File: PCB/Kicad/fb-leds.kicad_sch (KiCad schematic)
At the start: 52 parts, among them Q1 MMBTA05L, Q2 MMBTA05L, Q3 MMBTA05L, Q4 MMBTA05L

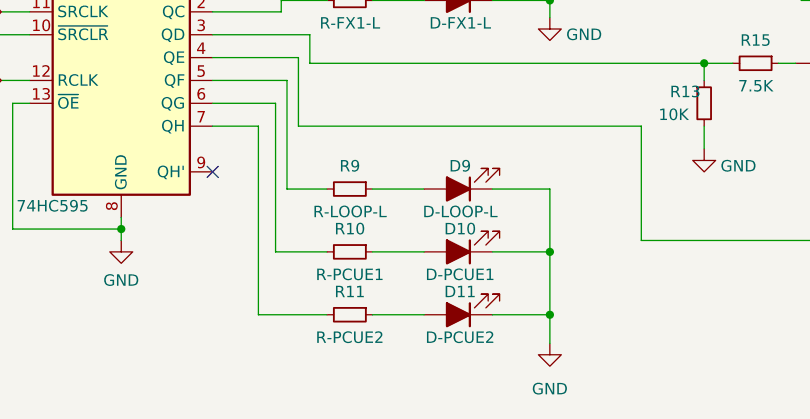
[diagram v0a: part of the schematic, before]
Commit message: routing WIP
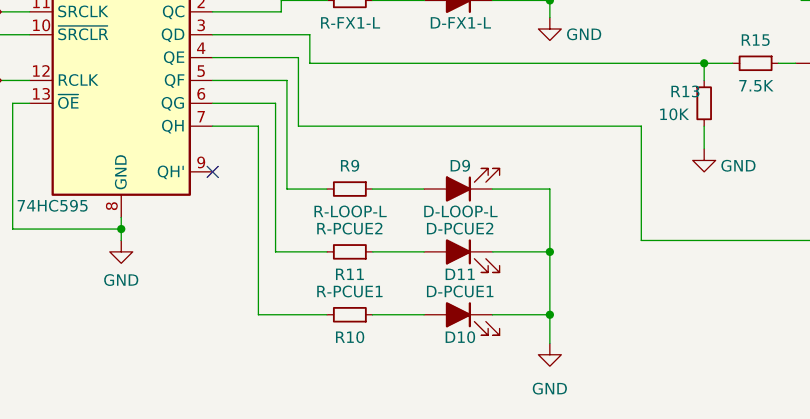
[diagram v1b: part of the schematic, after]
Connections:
- net at SR-FB-LEFT1.6 (QG): now also R11.2; no longer R10.2
- net at SR-FB-LEFT1.7 (QH): now also R10.2; no longer R11.2
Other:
- moved on the sheet: D10, D11, R10, R11
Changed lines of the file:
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@@
     (pin "2")
   )
-  (symbol (lib_id "Device:R_Small") (at 124.46 161.925 270) (unit 1)
-    (in_bom yes) (on_board yes)
-    (property "Reference" "R10" (id 0) (at 124.46 159.385 90))
-    (property "Value" "R-PCUE1" (id 1) (at 124.46 164.465 90))
+  (symbol (lib_id "Device:R_Small") (at 124.46 161.925 270) (mirror x) (unit 1)
+    (in_bom yes) (on_board yes)
+    (property "Reference" "R11" (id 0) (at 124.46 164.465 90))
+    (property "Value" "R-PCUE2" (id 1) (at 124.46 159.385 90))
     (property "Footprint" "Library:R_1206_3216Metric_Pad1.30x1.75mm_HandSolder" (id 2) (at 124.46 161.925 0)
       (effects (font (size 1.27 1.27)) hide)
@@
     (pin "2")
   )
-  (symbol (lib_id "Device:R_Small") (at 124.46 168.91 270) (unit 1)
-    (in_bom yes) (on_board yes)
-    (property "Reference" "R11" (id 0) (at 124.46 166.37 90))
-    (property "Value" "R-PCUE2" (id 1) (at 124.46 171.45 90))
+  (symbol (lib_id "Device:R_Small") (at 124.46 168.91 270) (mirror x) (unit 1)
+    (in_bom yes) (on_board yes)
+    (property "Reference" "R10" (id 0) (at 124.46 171.45 90))
+    (property "Value" "R-PCUE1" (id 1) (at 124.46 166.37 90))
     (property "Footprint" "Library:R_1206_3216Metric_Pad1.30x1.75mm_HandSolder" (id 2) (at 124.46 168.91 0)
       (effects (font (size 1.27 1.27)) hide)
@@
     (pin "2")
   )
-  (symbol (lib_id "Device:LED_Filled") (at 136.525 161.925 180) (unit 1)
-    (in_bom yes) (on_board yes)
-    (property "Reference" "D10" (id 0) (at 136.7155 159.385 0))
-    (property "Value" "D-PCUE1" (id 1) (at 136.7155 164.465 0))
+  (symbol (lib_id "Device:LED_Filled") (at 136.525 161.925 0) (mirror y) (unit 1)
+    (in_bom yes) (on_board yes)
+    (property "Reference" "D11" (id 0) (at 136.7155 164.465 0))
+    (property "Value" "D-PCUE2" (id 1) (at 136.7155 159.385 0))
     (property "Footprint" "Library:LED_1206_3216Metric_Pad1.42x1.75mm_HandSolder" (id 2) (at 136.525 161.925 0)
       (effects (font (size 1.27 1.27)) hide)
@@
     (pin "2")
   )
-  (symbol (lib_id "Device:LED_Filled") (at 136.525 168.91 180) (unit 1)
-    (in_bom yes) (on_board yes)
-    (property "Reference" "D11" (id 0) (at 136.7155 166.37 0))
-    (property "Value" "D-PCUE2" (id 1) (at 136.7155 171.45 0))
+  (symbol (lib_id "Device:LED_Filled") (at 136.525 168.91 0) (mirror y) (unit 1)
+    (in_bom yes) (on_board yes)
+    (property "Reference" "D10" (id 0) (at 136.7155 171.45 0))
+    (property "Value" "D-PCUE1" (id 1) (at 136.7155 166.37 0))
     (property "Footprint" "Library:LED_1206_3216Metric_Pad1.42x1.75mm_HandSolder" (id 2) (at 136.525 168.91 0)
       (effects (font (size 1.27 1.27)) hide)

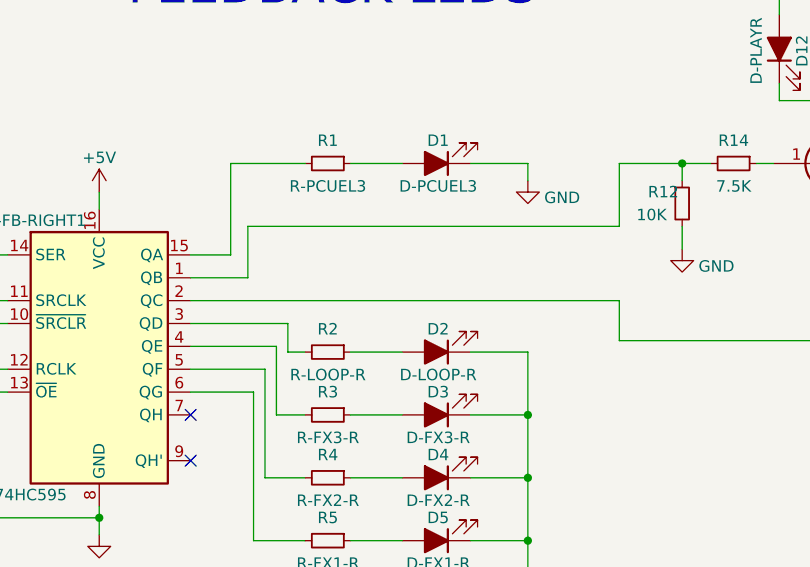
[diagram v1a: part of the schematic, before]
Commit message: routing WIP
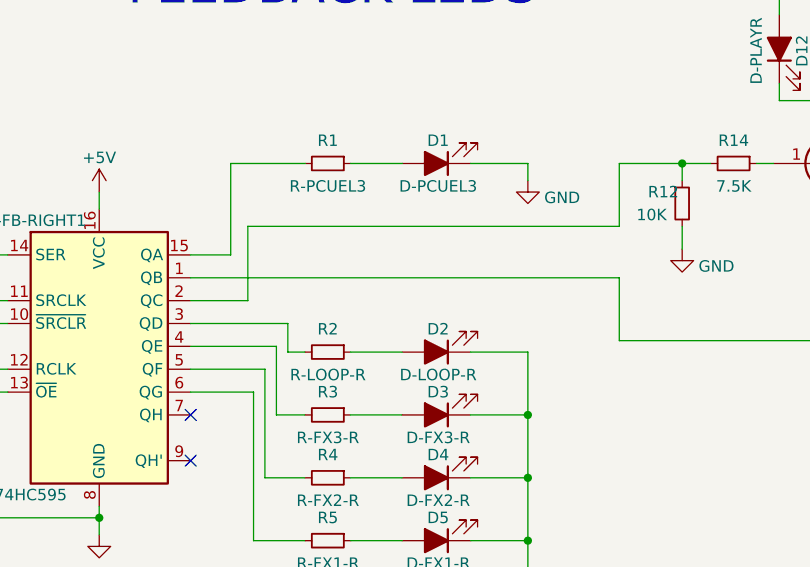
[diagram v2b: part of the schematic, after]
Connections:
- net at R12.1, R14.2: now also SR-FB-RIGHT1.2 (QC); no longer SR-FB-RIGHT1.1 (QB)
- net at R18.1, R20.2: now also SR-FB-RIGHT1.1 (QB); no longer SR-FB-RIGHT1.2 (QC)
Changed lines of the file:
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@@
     (stroke (width 0) (type solid) (color 0 0 0 0))
   )
-  (wire (pts (xy 109.22 66.04) (xy 115.57 66.04))
-    (stroke (width 0) (type solid) (color 0 0 0 0))
-  )
-  (wire (pts (xy 109.22 68.58) (xy 156.845 68.58))
-    (stroke (width 0) (type solid) (color 0 0 0 0))
+  (wire (pts (xy 109.22 68.58) (xy 115.57 68.58))
+    (stroke (width 0) (type default) (color 0 0 0 0))
   )
   (wire (pts (xy 109.22 71.12) (xy 120.015 71.12))
@@
     (stroke (width 0) (type solid) (color 0 0 0 0))
   )
+  (wire (pts (xy 115.57 60.325) (xy 115.57 68.58))
+    (stroke (width 0) (type solid) (color 0 0 0 0))
+  )
   (wire (pts (xy 115.57 60.325) (xy 156.845 60.325))
     (stroke (width 0) (type solid) (color 0 0 0 0))
   )
-  (wire (pts (xy 115.57 66.04) (xy 115.57 60.325))
-    (stroke (width 0) (type solid) (color 0 0 0 0))
-  )
   (wire (pts (xy 115.57 127) (xy 121.92 127))
     (stroke (width 0) (type solid) (color 0 0 0 0))
@@
     (stroke (width 0) (type solid) (color 0 0 0 0))
   )
-  (wire (pts (xy 156.845 68.58) (xy 156.845 73.025))
-    (stroke (width 0) (type solid) (color 0 0 0 0))
-  )
+  (wire (pts (xy 156.845 66.04) (xy 109.22 66.04))
+    (stroke (width 0) (type default) (color 0 0 0 0))
+  )
+  (wire (pts (xy 156.845 66.04) (xy 156.845 73.025))
+    (stroke (width 0) (type solid) (color 0 0 0 0))
+  )

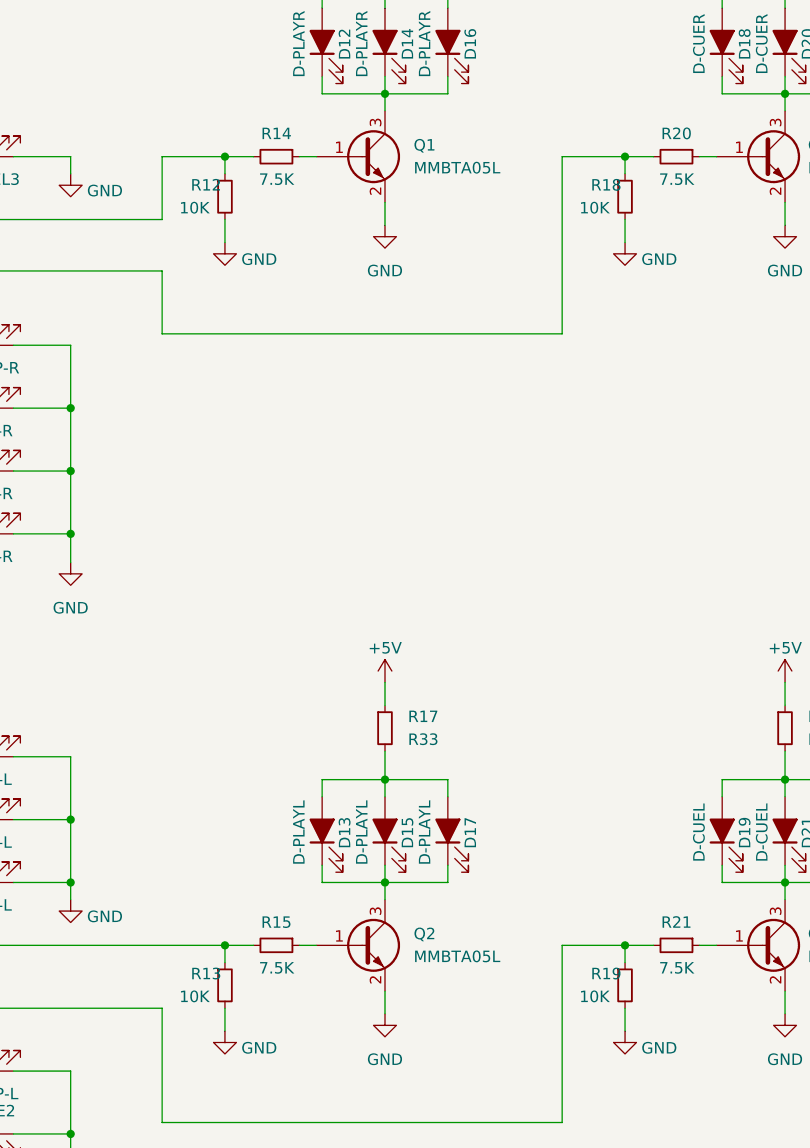
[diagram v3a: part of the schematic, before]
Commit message: routes finished
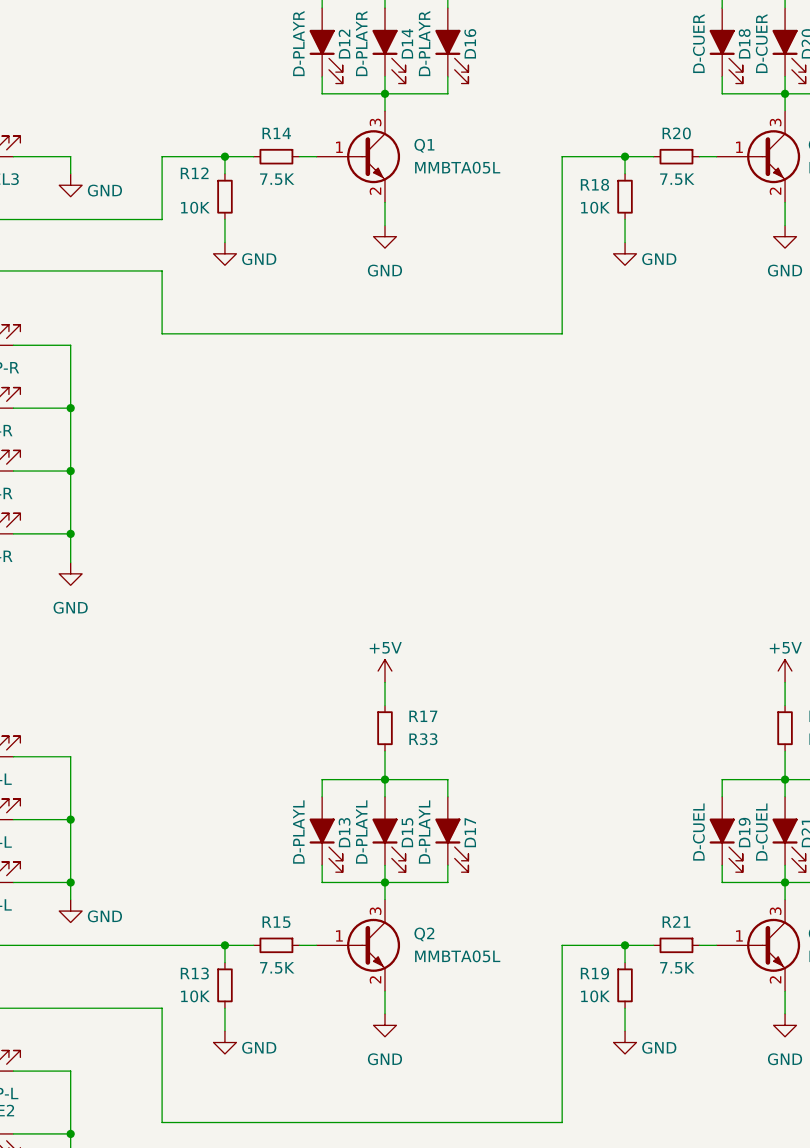
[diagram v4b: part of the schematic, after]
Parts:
- D1, D10, D11, D12, D13, D14, D15, D16, D17, D18, D19, D2, D20, D21, D22, D23, D3, D4, D5, D6, D7, D8, D9: footprint Library:LED_1206_3216Metric_Pad1.42x1.75mm_HandSolder -> LED_SMD:LED_1206_3216Metric_Pad1.42x1.75mm_HandSolder
